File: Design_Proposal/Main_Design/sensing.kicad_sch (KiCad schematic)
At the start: 13 parts, among them IC2 LM75AD,118, J12 Conn_01x03_Male, J13 Conn_01x05_Male

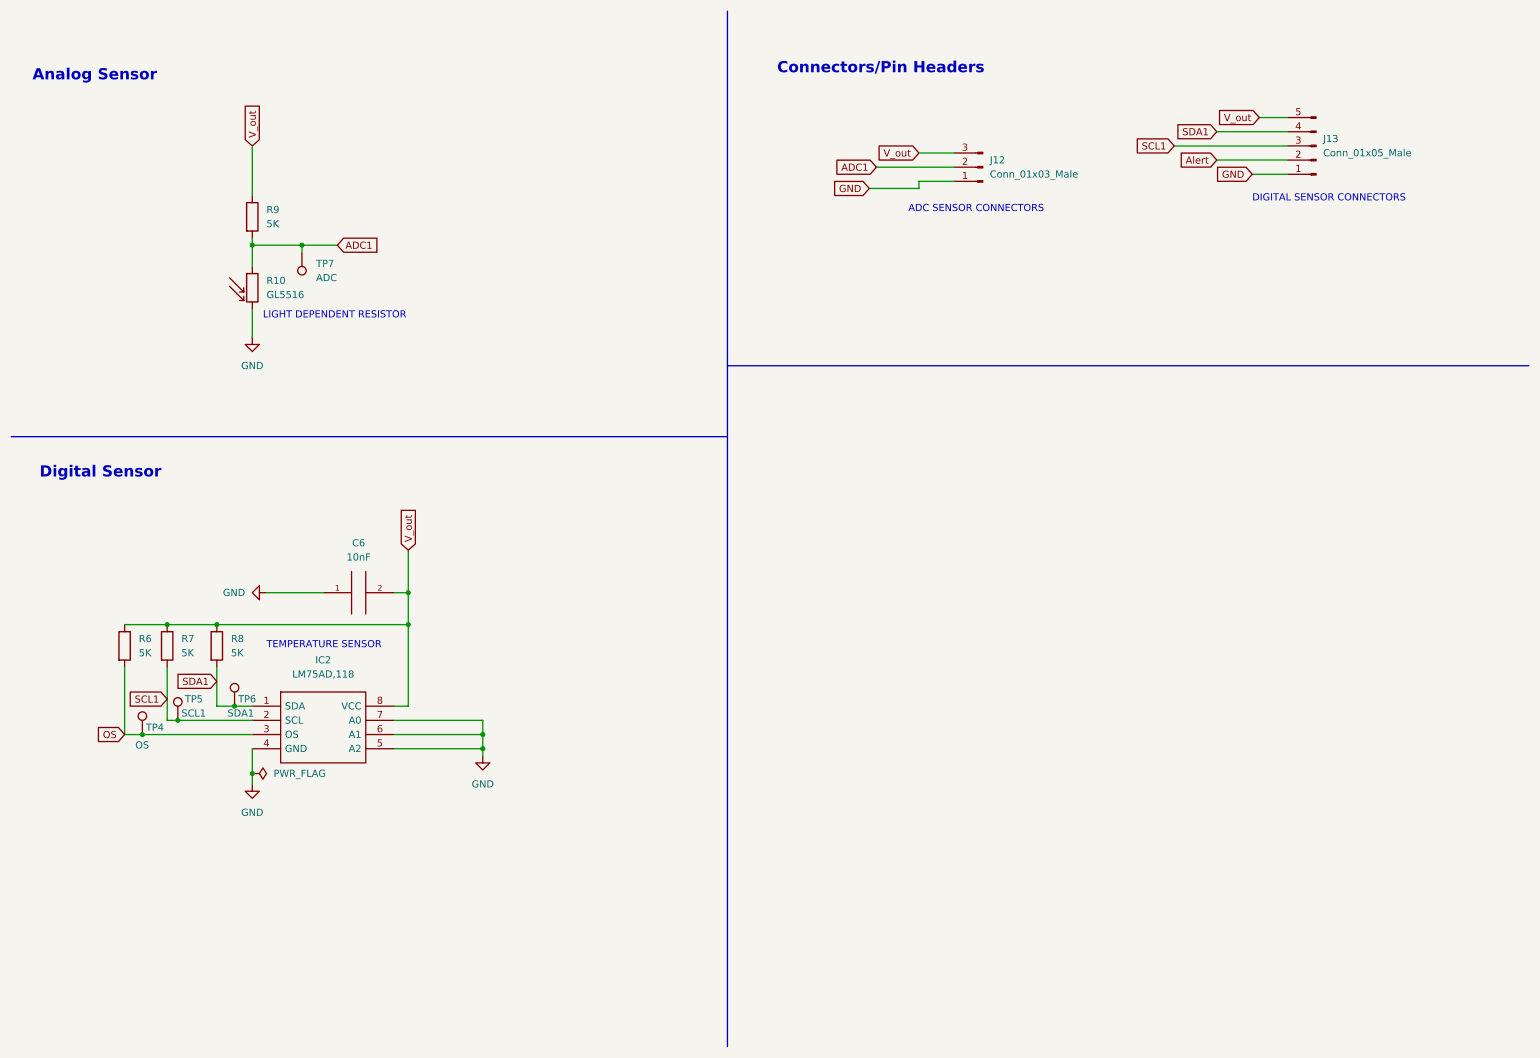
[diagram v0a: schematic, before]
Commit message: update
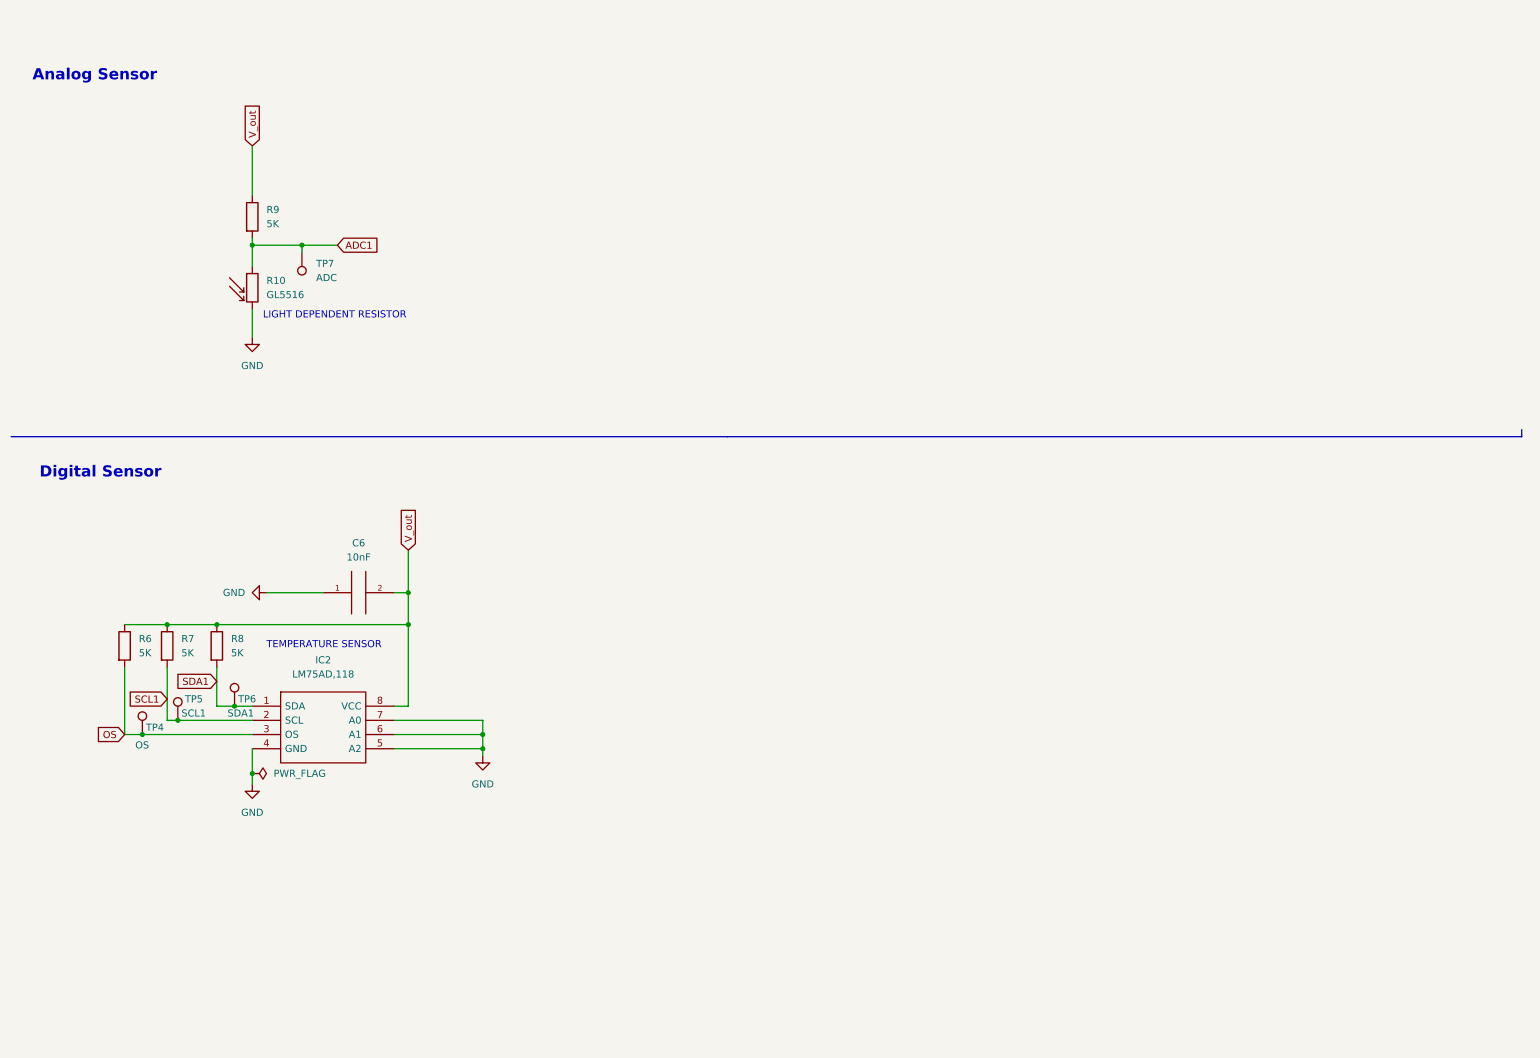
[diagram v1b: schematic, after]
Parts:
- removed J12: Conn_01x03_Male, Connector_PinHeader_2.54mm:PinHeader_1x03_P2.54mm_Vertical, symbol Connector:Conn_01x03_Male
- removed J13: Conn_01x05_Male, Connector_PinHeader_2.54mm:PinHeader_1x05_P2.54mm_Vertical, symbol Connector:Conn_01x05_Male
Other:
- note removed: "ADC SENSOR CONNECTORS"
- note removed: "Connectors/Pin Headers"
- note removed: "DIGITAL SENSOR CONNECTORS"
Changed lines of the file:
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@@
-    (stroke (width 0) (type default) (color 0 0 0 0))
-  )
-  (wire (pts (xy 236.22 31.75) (xy 241.3 31.75))
     (stroke (width 0) (type default) (color 0 0 0 0))
   )
@@
     (stroke (width 0) (type default) (color 0 0 0 0))
   )
-  (wire (pts (xy 166.37 44.45) (xy 175.26 44.45))
-    (stroke (width 0) (type default) (color 0 0 0 0))
-  )
-  (polyline (pts (xy 140.97 76.2) (xy 284.48 76.2))
-    (stroke (width 0) (type default) (color 0 0 0 0))
-  )
   (wire (pts (xy 81.28 116.84) (xy 83.82 116.84))
     (stroke (width 0) (type default) (color 0 0 0 0))
@@
     (stroke (width 0) (type default) (color 0 0 0 0))
   )
-  (wire (pts (xy 175.26 43.18) (xy 181.61 43.18))
-    (stroke (width 0) (type default) (color 0 0 0 0))
-  )
   (wire (pts (xy 83.82 109.22) (xy 83.82 116.84))
     (stroke (width 0) (type default) (color 0 0 0 0))
@@
     (stroke (width 0) (type default) (color 0 0 0 0))
   )
-  (wire (pts (xy 228.6 34.29) (xy 241.3 34.29))
-    (stroke (width 0) (type default) (color 0 0 0 0))
-  )
-  (wire (pts (xy 234.95 41.91) (xy 241.3 41.91))
+  (polyline (pts (xy 283.21 87.63) (xy 283.21 88.9))
     (stroke (width 0) (type default) (color 0 0 0 0))
   )
@@
     (stroke (width 0) (type default) (color 0 0 0 0))
   )
+  (polyline (pts (xy 140.97 88.9) (xy 283.21 88.9))
+    (stroke (width 0) (type default) (color 0 0 0 0))
+  )
   (wire (pts (xy 55.88 149.225) (xy 55.88 151.13))
     (stroke (width 0) (type default) (color 0 0 0 0))
@@
     (stroke (width 0) (type default) (color 0 0 0 0))
   )
-  (wire (pts (xy 167.64 40.64) (xy 181.61 40.64))
-    (stroke (width 0) (type default) (color 0 0 0 0))
-  )
   (wire (pts (xy 55.88 66.04) (xy 55.88 71.12))
     (stroke (width 0) (type default) (color 0 0 0 0))
   )
-  (wire (pts (xy 175.26 38.1) (xy 181.61 38.1))
-    (stroke (width 0) (type default) (color 0 0 0 0))
-  )
-  (wire (pts (xy 228.6 39.37) (xy 241.3 39.37))
-    (stroke (width 0) (type default) (color 0 0 0 0))
-  )
-  (polyline (pts (xy 140.97 88.9) (xy 140.97 198.12))
-    (stroke (width 0) (type default) (color 0 0 0 0))
-  )
   (wire (pts (xy 40.64 139.7) (xy 40.64 130.175))
     (stroke (width 0) (type default) (color 0 0 0 0))
@@
     (stroke (width 0) (type default) (color 0 0 0 0))
   )
-  (polyline (pts (xy 140.97 12.7) (xy 140.97 88.9))
-    (stroke (width 0) (type default) (color 0 0 0 0))
-  )
   (wire (pts (xy 55.88 54.61) (xy 55.88 58.42))
-    (stroke (width 0) (type default) (color 0 0 0 0))
-  )
-  (wire (pts (xy 175.26 44.45) (xy 175.26 43.18))
-    (stroke (width 0) (type default) (color 0 0 0 0))
-  )
-  (wire (pts (xy 220.98 36.83) (xy 241.3 36.83))
     (stroke (width 0) (type default) (color 0 0 0 0))
   )
@@
   )
   (text "LIGHT DEPENDENT RESISTOR" (at 57.785 67.945 0)
-    (effects (font (size 1.27 1.27)) (justify left bottom))
-  )
-  (text "Connectors/Pin Headers" (at 149.86 24.13 0)
-    (effects (font (size 2 2) bold) (justify left bottom))
-  )
-  (text "ADC SENSOR CONNECTORS\n" (at 173.355 48.895 0)
-    (effects (font (size 1.27 1.27)) (justify left bottom))
-  )
-  (text "DIGITAL SENSOR CONNECTORS\n" (at 234.95 46.99 0)
     (effects (font (size 1.27 1.27)) (justify left bottom))
   )
@@
     )
   )
-  (global_label "ADC1" (shape input) (at 167.64 40.64 180) (fields_autoplaced)
-    (effects (font (size 1.27 1.27)) (justify right))
-    (property "Intersheet References" "${INTERSHEET_REFS}" (id 0) (at 160.3888 40.7194 0)
-      (effects (font (size 1.27 1.27)) (justify right) hide)
-    )
-  )
-  (global_label "V_out" (shape input) (at 236.22 31.75 180) (fields_autoplaced)
-    (effects (font (size 1.27 1.27)) (justify right))
-    (property "Intersheet References" "${INTERSHEET_REFS}" (id 0) (at 228.7269 31.6706 0)
-      (effects (font (size 1.27 1.27)) (justify right) hide)
-    )
-  )
-  (global_label "Alert" (shape input) (at 228.6 39.37 180) (fields_autoplaced)
-    (effects (font (size 1.27 1.27)) (justify right))
-    (property "Intersheet References" "${INTERSHEET_REFS}" (id 0) (at 221.8326 39.4494 0)
-      (effects (font (size 1.27 1.27)) (justify right) hide)
-    )
-  )
   (global_label "SCL1" (shape input) (at 40.64 135.89 180) (fields_autoplaced)
     (effects (font (size 1.27 1.27)) (justify right))
@@
     )
   )
-  (global_label "V_out" (shape input) (at 175.26 38.1 180) (fields_autoplaced)
-    (effects (font (size 1.27 1.27)) (justify right))
-    (property "Intersheet References" "${INTERSHEET_REFS}" (id 0) (at 167.7669 38.0206 0)
-      (effects (font (size 1.27 1.27)) (justify right) hide)
-    )
-  )
-  (global_label "GND" (shape input) (at 234.95 41.91 180) (fields_autoplaced)
-    (effects (font (size 1.27 1.27)) (justify right))
-    (property "Intersheet References" "${INTERSHEET_REFS}" (id 0) (at 228.6664 41.9894 0)
-      (effects (font (size 1.27 1.27)) (justify right) hide)
-    )
-  )
-  (global_label "SDA1" (shape input) (at 228.6 34.29 180) (fields_autoplaced)
-    (effects (font (size 1.27 1.27)) (justify right))
-    (property "Intersheet References" "${INTERSHEET_REFS}" (id 0) (at 221.4093 34.3694 0)
-      (effects (font (size 1.27 1.27)) (justify right) hide)
-    )
-  )
-  (global_label "SCL1" (shape input) (at 220.98 36.83 180) (fields_autoplaced)
-    (effects (font (size 1.27 1.27)) (justify right))
-    (property "Intersheet References" "${INTERSHEET_REFS}" (id 0) (at 213.8498 36.9094 0)
-      (effects (font (size 1.27 1.27)) (justify right) hide)
-    )
-  )
-  (global_label "GND" (shape input) (at 166.37 44.45 180) (fields_autoplaced)
-    (effects (font (size 1.27 1.27)) (justify right))
-    (property "Intersheet References" "${INTERSHEET_REFS}" (id 0) (at 160.0864 44.3706 0)
-      (effects (font (size 1.27 1.27)) (justify right) hide)
-    )
-  )
   (symbol (lib_id "power:GND") (at 55.88 151.13 0) (unit 1)
     (in_bom yes) (on_board yes) (fields_autoplaced)
-    (property "Reference" "#PWR025" (id 0) (at 55.88 157.48 0)
+    (property "Reference" "#PWR024" (id 0) (at 55.88 157.48 0)
       (effects (font (size 1.27 1.27)) hide)
     )
@@
   (symbol (lib_id "power:GND") (at 58.42 116.84 270) (unit 1)
     (in_bom yes) (on_board yes) (fields_autoplaced)
-    (property "Reference" "#PWR026" (id 0) (at 52.07 116.84 0)
+    (property "Reference" "#PWR025" (id 0) (at 52.07 116.84 0)
       (effects (font (size 1.27 1.27)) hide)
     )
@@
     (pin "2")
   )
-  (symbol (lib_id "Connector:Conn_01x05_Male") (at 246.38 36.83 180) (unit 1)
-    (in_bom yes) (on_board yes) (fields_autoplaced)
-    (property "Reference" "J13" (id 0) (at 247.65 35.5599 0)
-      (effects (font (size 1.27 1.27)) (justify right))
-    )
-    (property "Value" "Conn_01x05_Male" (id 1) (at 247.65 38.0999 0)
-      (effects (font (size 1.27 1.27)) (justify right))
-    )
-    (property "Footprint" "Connector_PinHeader_2.54mm:PinHeader_1x05_P2.54mm_Vertical" (id 2) (at 246.38 36.83 0)
-      (effects (font (size 1.27 1.27)) hide)
-    )
-    (property "Datasheet" "~" (id 3) (at 246.38 36.83 0)
-      (effects (font (size 1.27 1.27)) hide)
-    )
-    (pin "1")
-    (pin "2")
-    (pin "3")
-    (pin "4")
-    (pin "5")
-  )
   (symbol (lib_id "power:GND") (at 55.88 71.12 0) (unit 1)
     (in_bom yes) (on_board yes) (fields_autoplaced)
-    (property "Reference" "#PWR024" (id 0) (at 55.88 77.47 0)
+    (property "Reference" "#PWR023" (id 0) (at 55.88 77.47 0)
       (effects (font (size 1.27 1.27)) hide)
     )
@@
     (pin "1")
   )
-  (symbol (lib_id "Connector:Conn_01x03_Male") (at 186.69 40.64 180) (unit 1)
-    (in_bom yes) (on_board yes) (fields_autoplaced)
-    (property "Reference" "J12" (id 0) (at 187.96 39.3699 0)
-      (effects (font (size 1.27 1.27)) (justify right))
-    )
-    (property "Value" "Conn_01x03_Male" (id 1) (at 187.96 41.9099 0)
-      (effects (font (size 1.27 1.27)) (justify right))
-    )
-    (property "Footprint" "Connector_PinHeader_2.54mm:PinHeader_1x03_P2.54mm_Vertical" (id 2) (at 186.69 40.64 0)
-      (effects (font (size 1.27 1.27)) hide)
-    )
-    (property "Datasheet" "~" (id 3) (at 186.69 40.64 0)
-      (effects (font (size 1.27 1.27)) hide)
-    )
-    (pin "1")
-    (pin "2")
-    (pin "3")
-  )
   (symbol (lib_id "power:GND") (at 97.155 146.05 0) (unit 1)
     (in_bom yes) (on_board yes) (fields_autoplaced)
-    (property "Reference" "#PWR027" (id 0) (at 97.155 152.4 0)
-      (effects (font (size 1.27 1.27)) hide)
-    )
+    (property "Reference" "#PWR026" (id 0) (at 97.155 152.4 0)
+      (effects (font (size 1.27 1.27)) hide)
+    )

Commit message: update
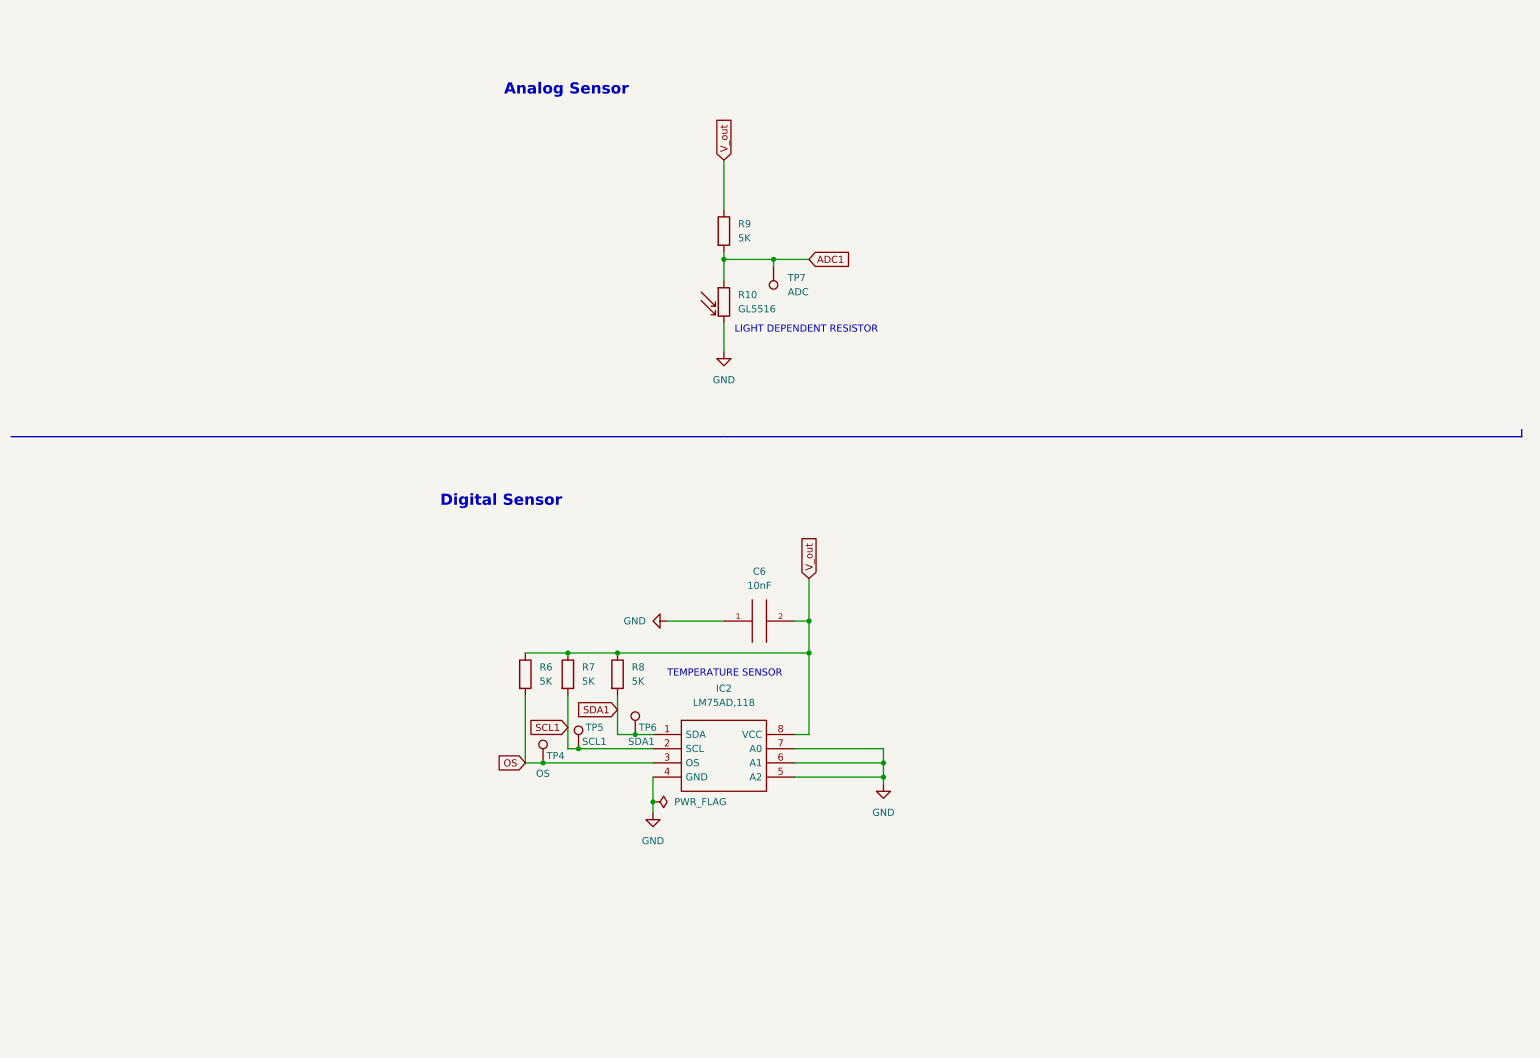
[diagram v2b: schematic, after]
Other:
- moved on the sheet: C6, IC2, R10, R6, R7, R8, R9, TP4, TP5, TP6, TP7
